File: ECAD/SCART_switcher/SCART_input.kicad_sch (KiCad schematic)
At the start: 33 parts, among them J1 SCART-F, Q1 BC847, Q2 BC847, U1 THS7374, U2 74AHC1G126, U3 74AHC1G126, U5 74AHC1G04, U6 TLV9002S, U7 74LVC2G66

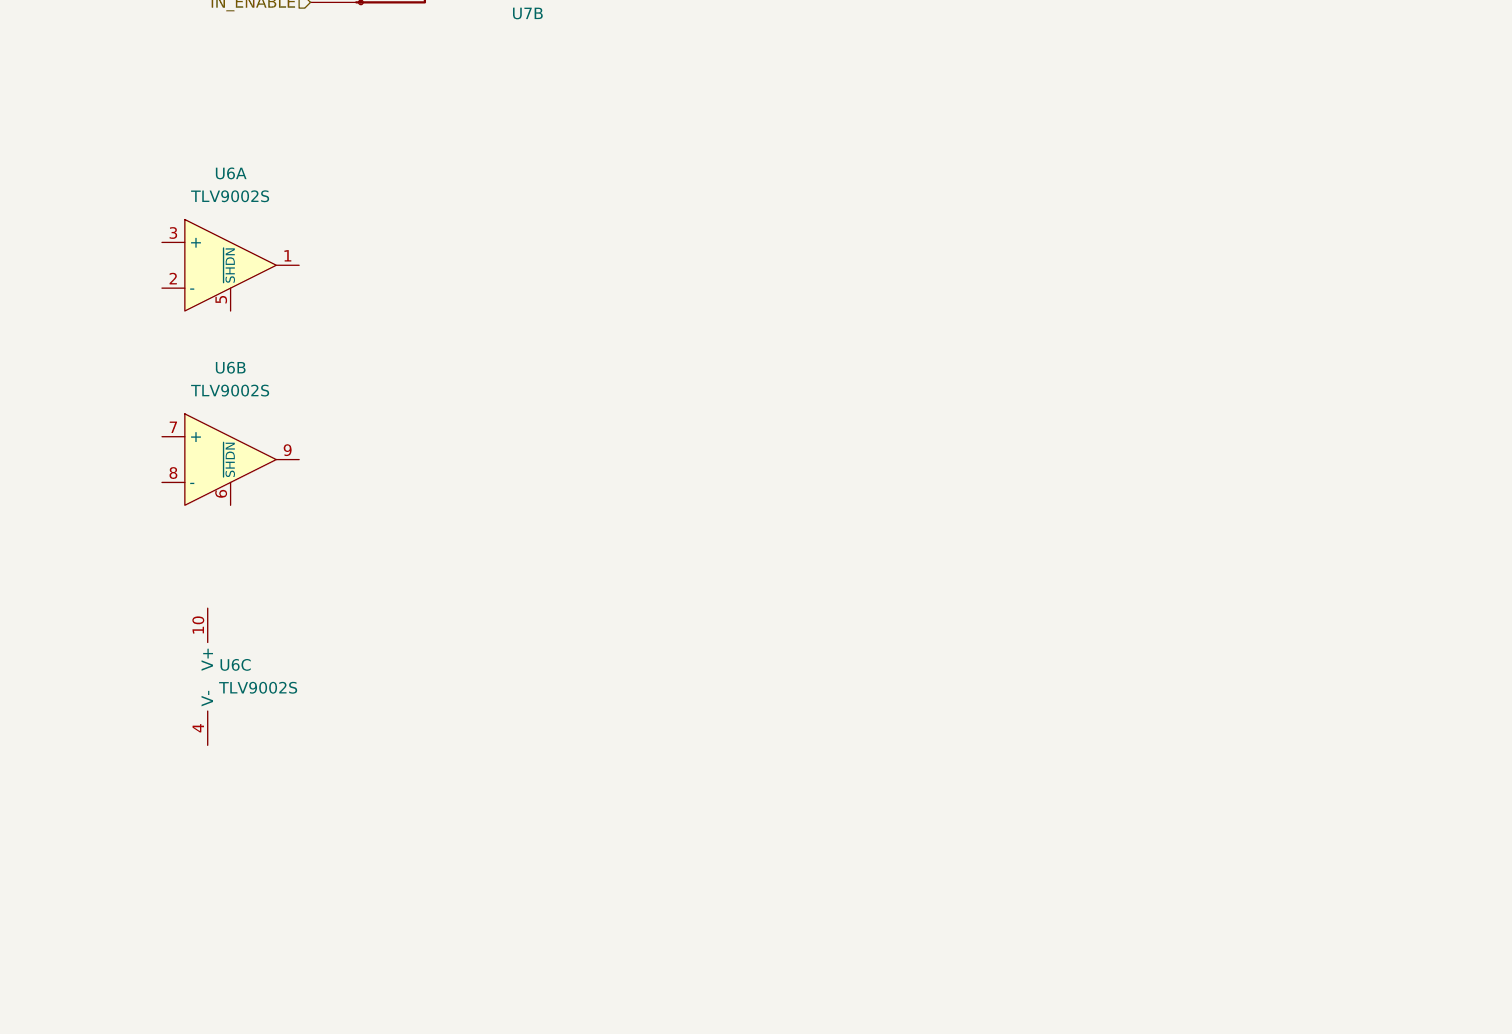
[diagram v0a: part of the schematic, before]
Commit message: progressed ECAD
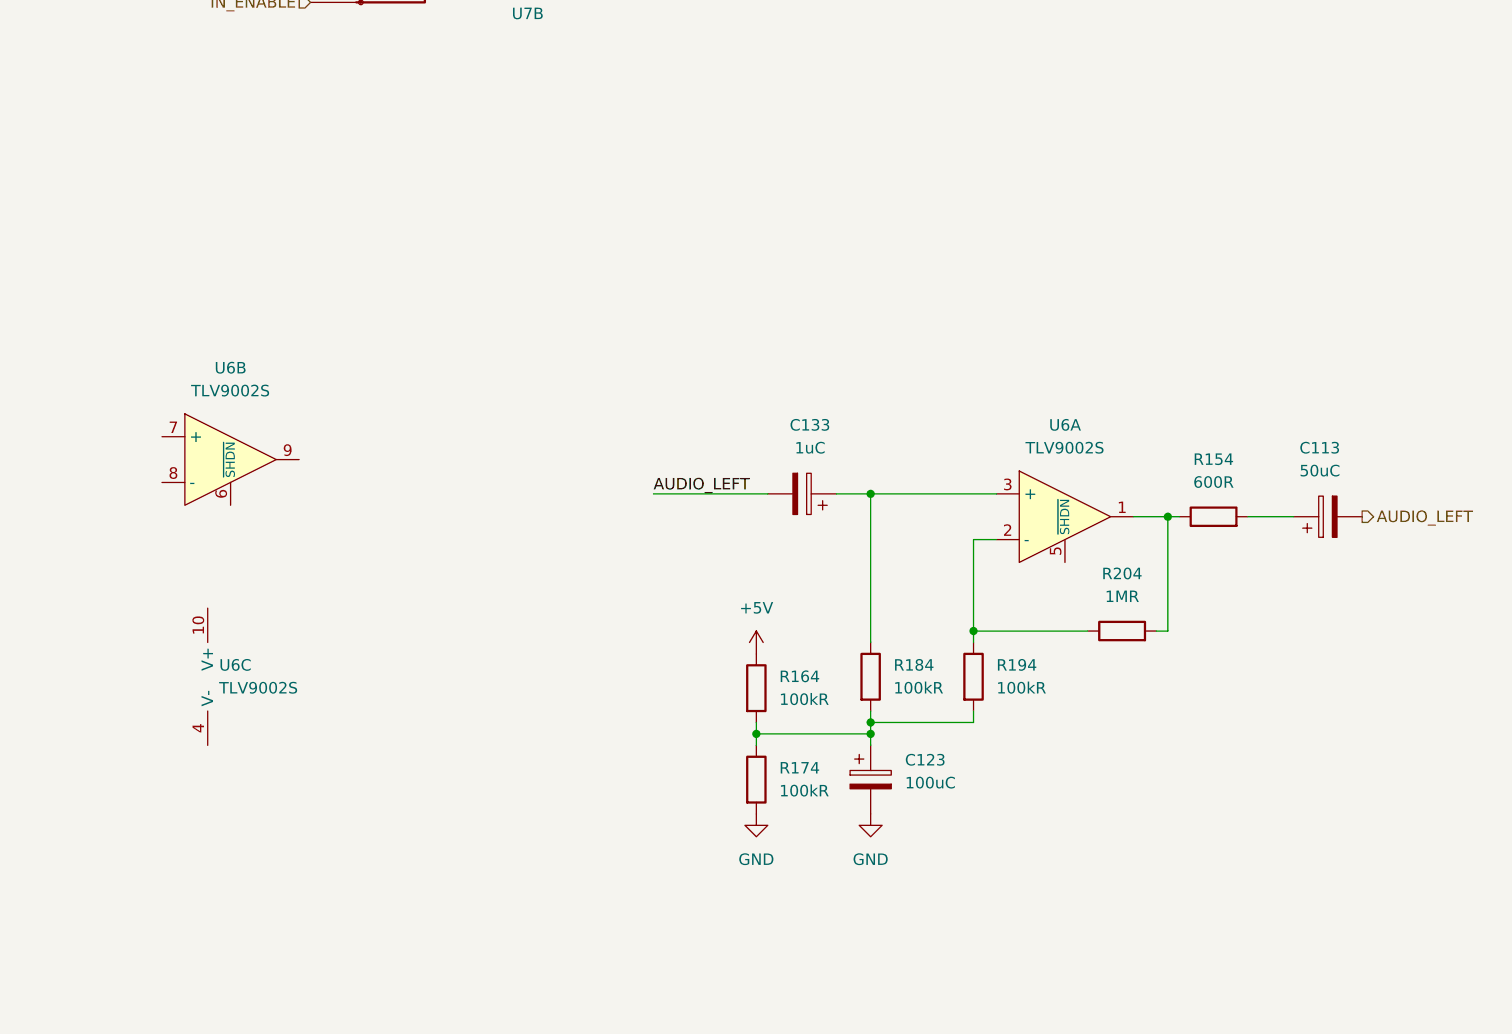
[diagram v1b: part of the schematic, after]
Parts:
- added C113: 50uC, symbol Device:C_Polarized
- added C123: 100uC, symbol Device:C_Polarized
- added C133: 1uC, symbol Device:C_Polarized
- added R154: 600R, symbol Device:R
- added R164, R174, R184, R194: 100kR, symbol Device:R
- added R204: 1MR, symbol Device:R
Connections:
- net +5V: now also R164.1
- net AUDIO_LEFT: now also C113.2, C133.2
- net GND: now also C123.2, R174.2
- net at U6.1: now also R154.1, R204.2
- net at U6.2 (-): now also R194.1, R204.1
- net at U6.3 (+): now also C133.1, R184.1
- new net: C123.1, R164.2, R174.1, R184.2, R194.2
- new net: C113.1, R154.2
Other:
- moved on the sheet: U6A

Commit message: Update SCART_input.kicad_sch
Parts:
- removed C133: 1uC, symbol Device:C_Polarized
- added C133, C183: 1uC, Capacitor_SMD:C_0805_2012Metric_Pad1.18x1.45mm_HandSolder, symbol Device:C
- added C144, C145: 100uC, symbol Device:C_Polarized
- added C88: 100nC, Capacitor_SMD:C_0805_2012Metric_Pad1.18x1.45mm_HandSolder, symbol Device:C
- added R214, R224: 10kR, Resistor_SMD:R_0805_2012Metric_Pad1.20x1.40mm_HandSolder, symbol Device:R
- added R225, R226: 10kR, symbol Device:R
- added R227, R228: 100kR, symbol Device:R
- added R229: 1MR, symbol Device:R
- added R230: 600R, symbol Device:R
- C113: value 50uC -> 100uC
- R164, R174: value 100kR -> 10kR
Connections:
- net +5V: now also U6.10 (V+), C88.1, R225.1
- net AUDIO_LEFT: now also C183.1, R214.1
- net AUDIO_RIGHT: now also C133.1, C145.2, R224.1
- net GND: now also U6.11 (V-), U6.4 (V-), C144.2, C88.2, R214.2, R224.2, R226.2
- net IN_ENABLE: now also U6.5 (~{SHDN}), U6.6 (~{SHDN})
- net at U6.7 (+): now also C133.2, R227.1
- net at U6.8 (-): now also R228.1, R229.1
- net at U6.9: now also R229.2, R230.1
- net at R184.1, U6.3 (+): now also C183.2
- new net: C144.1, R225.2, R226.1, R227.2, R228.2
- new net: C145.1, R230.2
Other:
- note added: "Audio signals buffer"
- note added: "virtual ground at 2.5V"
- moved on the sheet: C1, C113, C123, C2, C3, C4, C5, C6, C88, J1, Q1, Q2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
